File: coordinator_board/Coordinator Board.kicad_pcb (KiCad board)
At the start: 4 copper layers, 45.5 x 39.6 mm, 30 parts, among them J1 Conn_01x04, J2 Conn_01x04, J3 Conn_01x04, P4 SERIAL, SW1 Switch_SPDT_x2, SW2 Switch_DPST, U0 10118194, U1 LM3671, U2 CD74HC4050, U3 ESP-12E, U4 DIY-OLED-0.96, U5 SF303GJ26, U6 SN74LVC1T45, U7 SN74LVC1T45

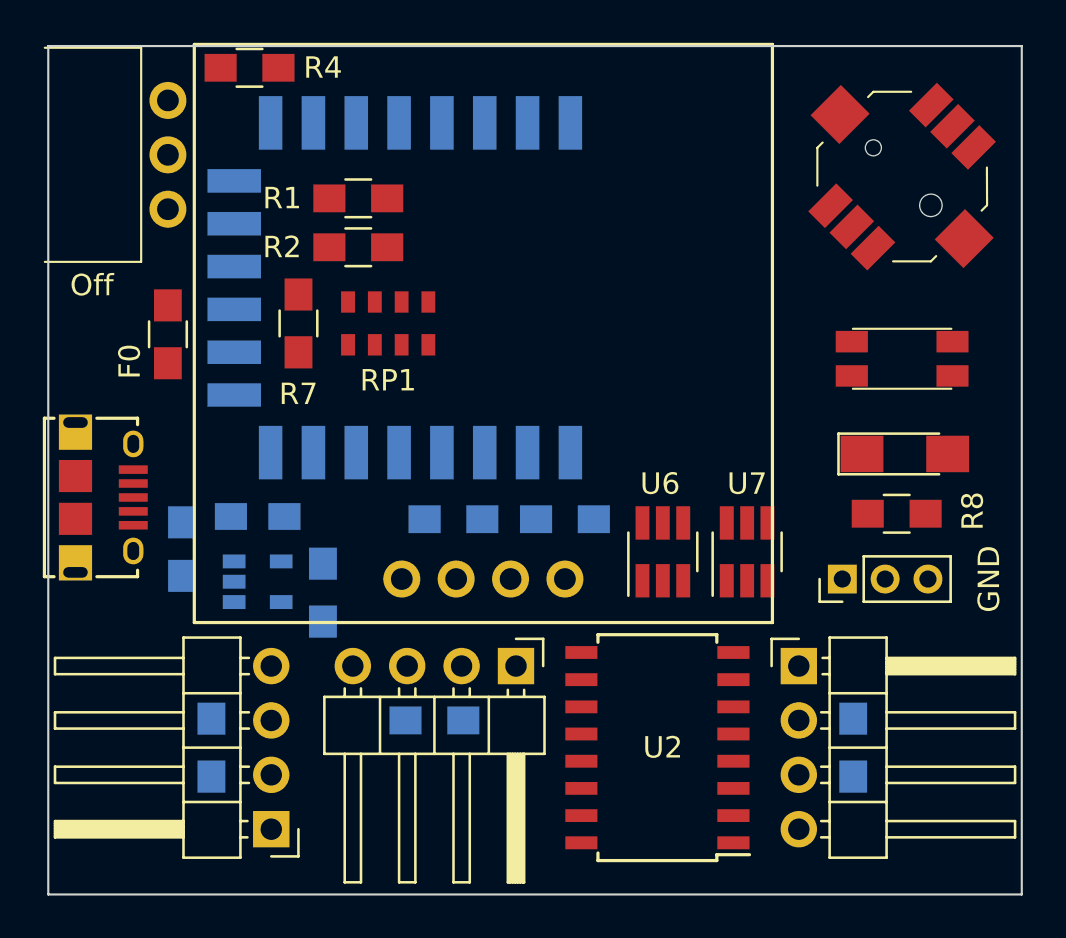
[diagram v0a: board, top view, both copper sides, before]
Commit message: Finished first draft of the board
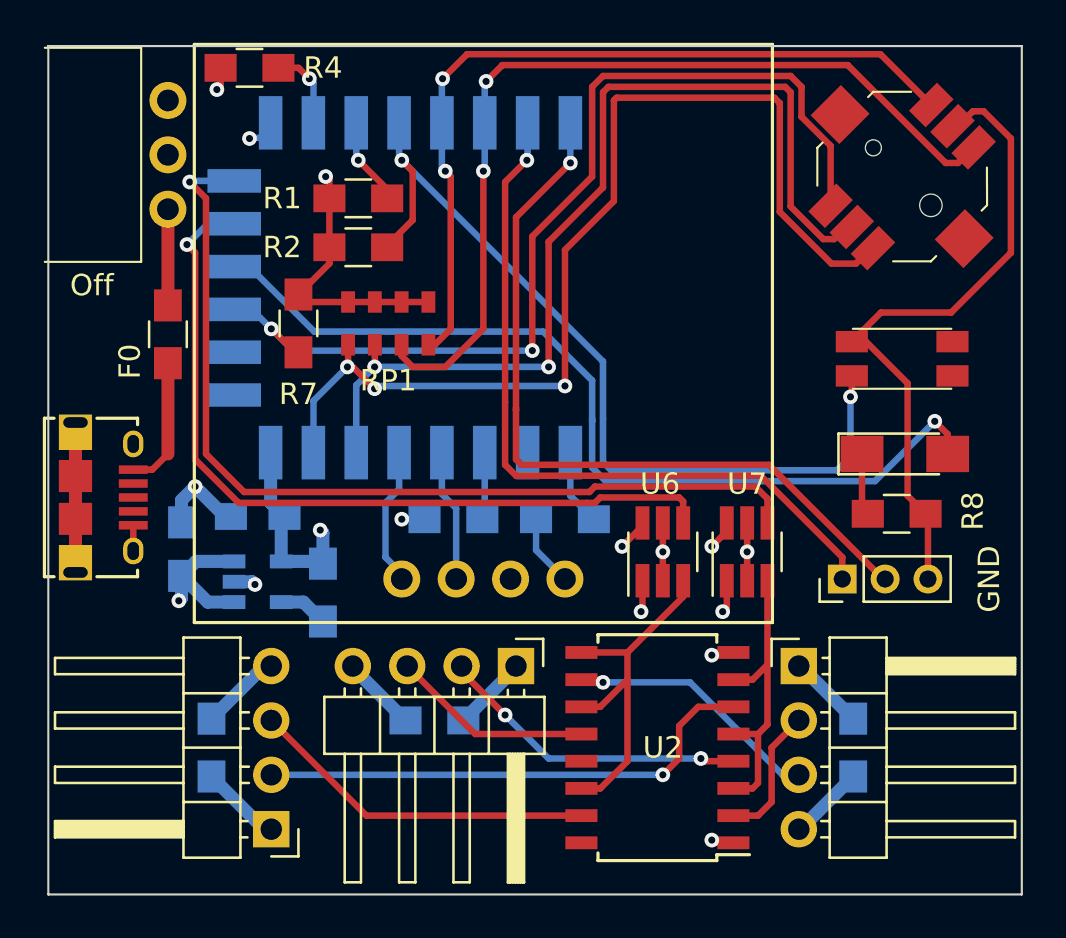
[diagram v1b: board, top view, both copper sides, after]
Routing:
- net GND: track 0.00 -> 63.9 mm, vias 0 -> 7
- net Net-(RP1-Pad1): track 0.00 -> 48.6 mm, vias 0 -> 3
- net Net-(R7-Pad2): track 0.00 -> 45.5 mm, vias 0 -> 2
- net Net-(U3-Pad22): track 0.00 -> 45.5 mm, vias 0 -> 1
- net Net-(RP1-Pad2): track 0.00 -> 44.7 mm, vias 0 -> 2
- net Net-(RP1-Pad3): track 0.00 -> 42.2 mm, vias 0 -> 2
- net Net-(D1-Pad2): track 0.00 -> 41.6 mm, vias 0 -> 1
- net Net-(U3-Pad21): track 0.00 -> 41.4 mm, vias 0 -> 1
- net Net-(R2-Pad1): track 0.00 -> 39.6 mm, vias 0 -> 2
- net Net-(RP1-Pad4): track 0.00 -> 37.5 mm, vias 0 -> 2
- net Net-(P4-Pad2): track 0.00 -> 35.7 mm, vias 0 -> 1
- net Net-(P4-Pad1): track 0.00 -> 34.3 mm, vias 0 -> 1
- net +3V3: track 0.00 -> 29.4 mm, vias 0 -> 5
- net Net-(J1-Pad2): track 0.00 -> 23.8 mm, vias 0 -> 1
- net +5V: track 0.00 -> 21.9 mm, vias 0 -> 4
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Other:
- rule pad_to_mask_clearance: 0 -> 0.0508
